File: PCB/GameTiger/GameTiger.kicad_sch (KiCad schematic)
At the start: 52 parts, among them J1 USB_B_Micro, U1 RP2040, U2 NCP1117-3.3_SOT223, U3 W25Q128JVS, U4 PAM8302A, Y1 ABLS-12MHZ-B4-T

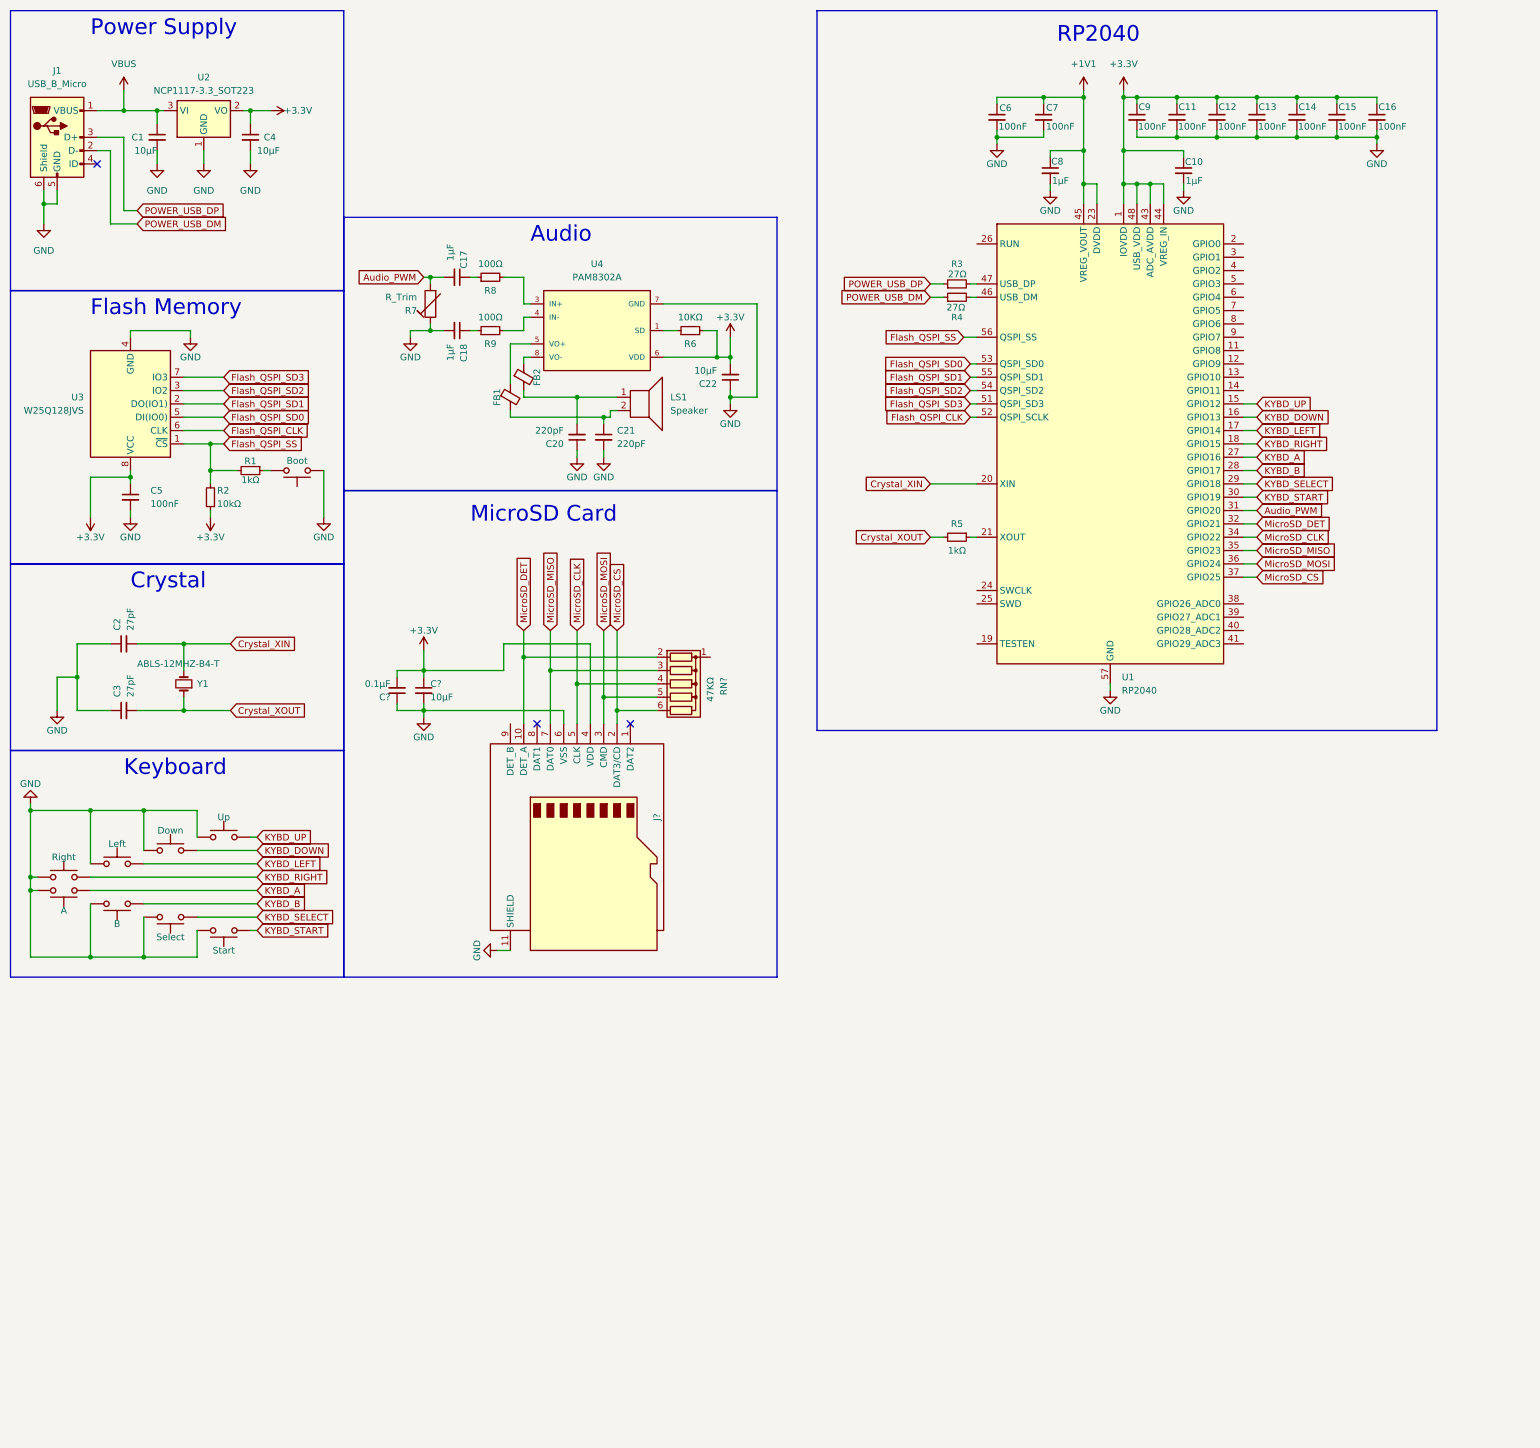
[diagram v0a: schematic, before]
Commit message: PCB Schematic for V2.0 is completed
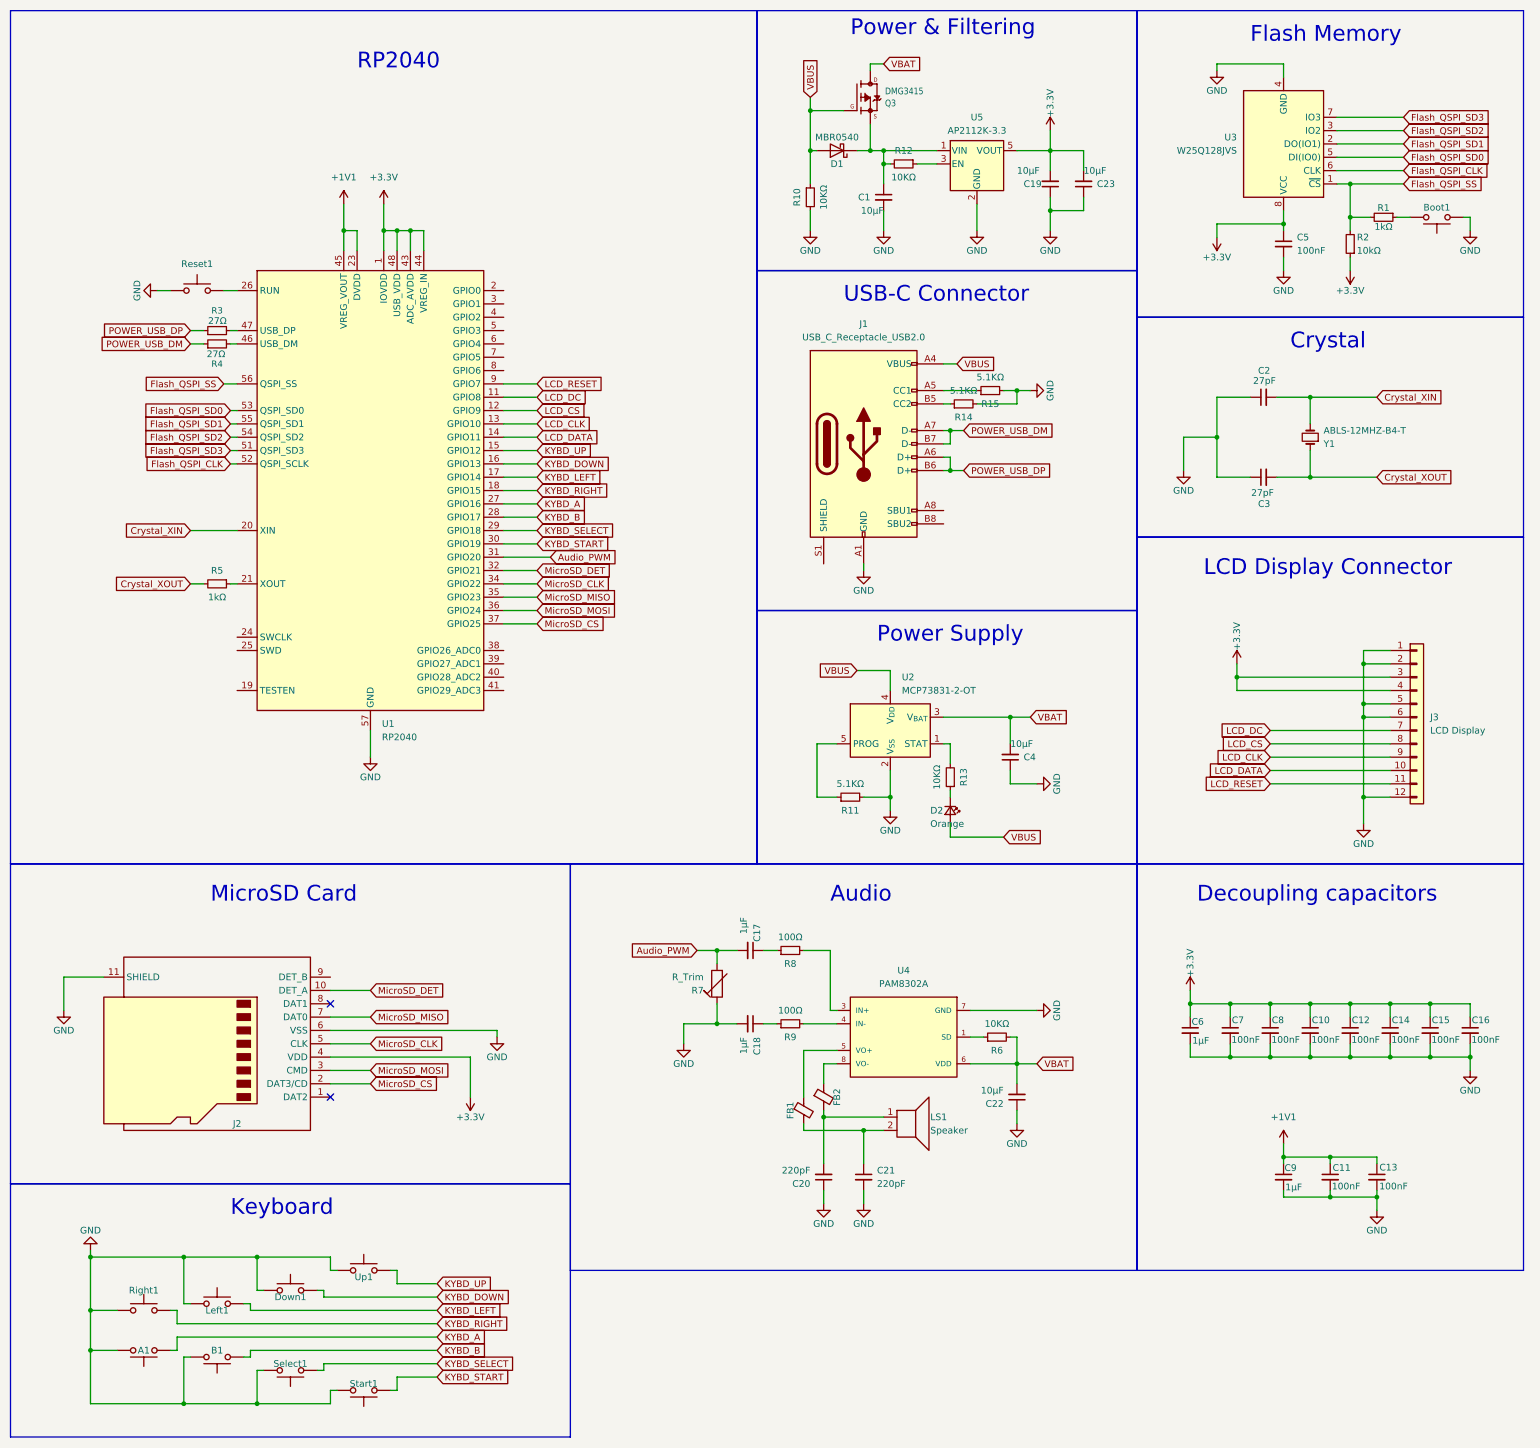
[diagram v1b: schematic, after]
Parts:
- removed C?: 10μF, symbol Device:C_Small
- removed C?: 0.1μF, symbol Device:C_Small
- removed J1: USB_B_Micro, symbol Connector:USB_B_Micro
- removed RN?: 47KΩ, Resistor_THT:R_Array_SIP6, symbol Device:R_Network05
- removed U2: NCP1117-3.3_SOT223, Package_TO_SOT_SMD:SOT-223-3_TabPin2, symbol Regulator_Linear:NCP1117-3.3_SOT223
- added C19, C23: 10μF, symbol Device:C_Small
- added D1: MBR0540, Diode_SMD:D_SOD-123, symbol Diode:MBR0540
- added D2: Orange, symbol Device:LED_Small
- added J1: USB_C_Receptacle_USB2.0, symbol Connector:USB_C_Receptacle_USB2.0
- added J3: LCD Display, symbol Connector_Generic:Conn_01x12
- added Q3: DMG3415, Adafruit Feather RP2040:SOT23-R, symbol Adafruit Feather RP2040-eagle-import:MOSFET-P
- added R10, R12, R13: 10KΩ, symbol Device:R_Small
- added R11, R14, R15: 5.1KΩ, symbol Device:R_Small
- added Reset1: SW_Push, symbol Switch:SW_Push
- added U2: MCP73831-2-OT, Package_TO_SOT_SMD:SOT-23-5, symbol Battery_Management:MCP73831-2-OT
- added U5: AP2112K-3.3, Package_TO_SOT_SMD:SOT-23-5, symbol Regulator_Linear:AP2112K-3.3
- C10, C8: value 1μF -> 100nF
- C6, C9: value 100nF -> 1μF
- gave numbers to parts that had none: 1
- renumbered A to A1, B to B1, Boot to Boot1, Down to Down1, Left to Left1, Right to Right1, Select to Select1, Start to Start1, Up to Up1
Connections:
- net +1V1: now also C11.1, C13.1, C9.1; no longer C6.1, C7.1, C8.1
- net +3.3V: now also C6.1, C7.1, C8.1, C19.2, C23.2, J3.3 (Pin_3), J3.4 (Pin_4), U5.5 (VOUT); no longer C11.1, C13.1, C22.2, C4.1, C9.1, R6.2, U4.6 (VDD)
- net GND: now also C4.1, C19.1, C23.1, J1.A1 (GND), J1.A12 (GND), J1.B1 (GND), J1.B12 (GND), J3.1 (Pin_1), J3.12 (Pin_12), J3.2 (Pin_2), J3.5 (Pin_5), J3.6 (Pin_6), R10.2, R11.2, R14.2, R15.2, Reset1.1, U2.2 (V_{SS}), U5.2 (GND); no longer C4.2
- net POWER_USB_DM: now also J1.A7 (D-), J1.B7 (D-)
- net POWER_USB_DP: now also J1.A6 (D+), J1.B6 (D+)
- net VBUS: now also D1.2 (A), D2.2 (A), J1.A4 (VBUS), J1.A9 (VBUS), J1.B4 (VBUS), J1.B9 (VBUS), Q3.1 (G), R10.1, U2.4 (V_{DD}); no longer C1.1
- net LCD_DC: now reaches U1.11 (GPIO8)
- net LCD_DC: now also J3.7 (Pin_7)
- net LCD_CS: now reaches U1.12 (GPIO9)
- net LCD_CS: now also J3.8 (Pin_8)
- net LCD_CLK: now reaches U1.13 (GPIO10)
- net LCD_CLK: now also J3.9 (Pin_9)
- net LCD_DATA: now reaches U1.14 (GPIO11)
- net LCD_DATA: now also J3.10 (Pin_10)
- net at U1.26 (RUN): now also Reset1.2
- net LCD_RESET: now reaches U1.9 (GPIO7)
- net LCD_RESET: now also J3.11 (Pin_11)
- new net: J1.B5 (CC2), R14.1
- new net: J1.A5 (CC1), R15.1
- new net: R12.1, U5.3 (EN)
- new net: C1.1, D1.1 (K), Q3.2 (S), R12.2, U5.1 (VIN)
- new net: R11.1, U2.5 (PROG)
- new net: D2.1 (K), R13.1
- new net: R13.2, U2.1 (STAT)
- new net VBAT: C22.2, C4.2, Q3.3 (D), R6.2, U2.3 (V_{BAT}), U4.6 (VDD)
- no-connect marks 3 -> 2
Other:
- note added: "Decoupling capacitors"
- note added: "LCD Display Connector"
- note added: "Power & Filtering"
- note added: "USB-C Connector"
- moved on the sheet: A1, B1, Boot1, C17, C18, C2, C20, C21, C22, C3, C5, Down1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
